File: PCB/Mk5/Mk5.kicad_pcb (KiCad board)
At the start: 2 copper layers, 197 x 253 mm, 40 parts, among them J1 KeyBoard 5,Rd,Ld,D7..0,Gnd, J2 PortB, J3 PortA, J4 COM: Gnd,Rx,Tx,Rts,Dcd,Cts,5v, J5 Conn_01x12, J6 Screw_Terminal_01x02, J7 Conn_01x06_Pin, SW1 SW_Push, U1 74LS92, U10 GAL20V8B-10, U11 GAL20V8B-10, U2 R65C02, U3 CD4059A, U4 EEPROM, U5 62256, U6 MC68B50, U7 R6522, U8 74LS573, U9 DS1813

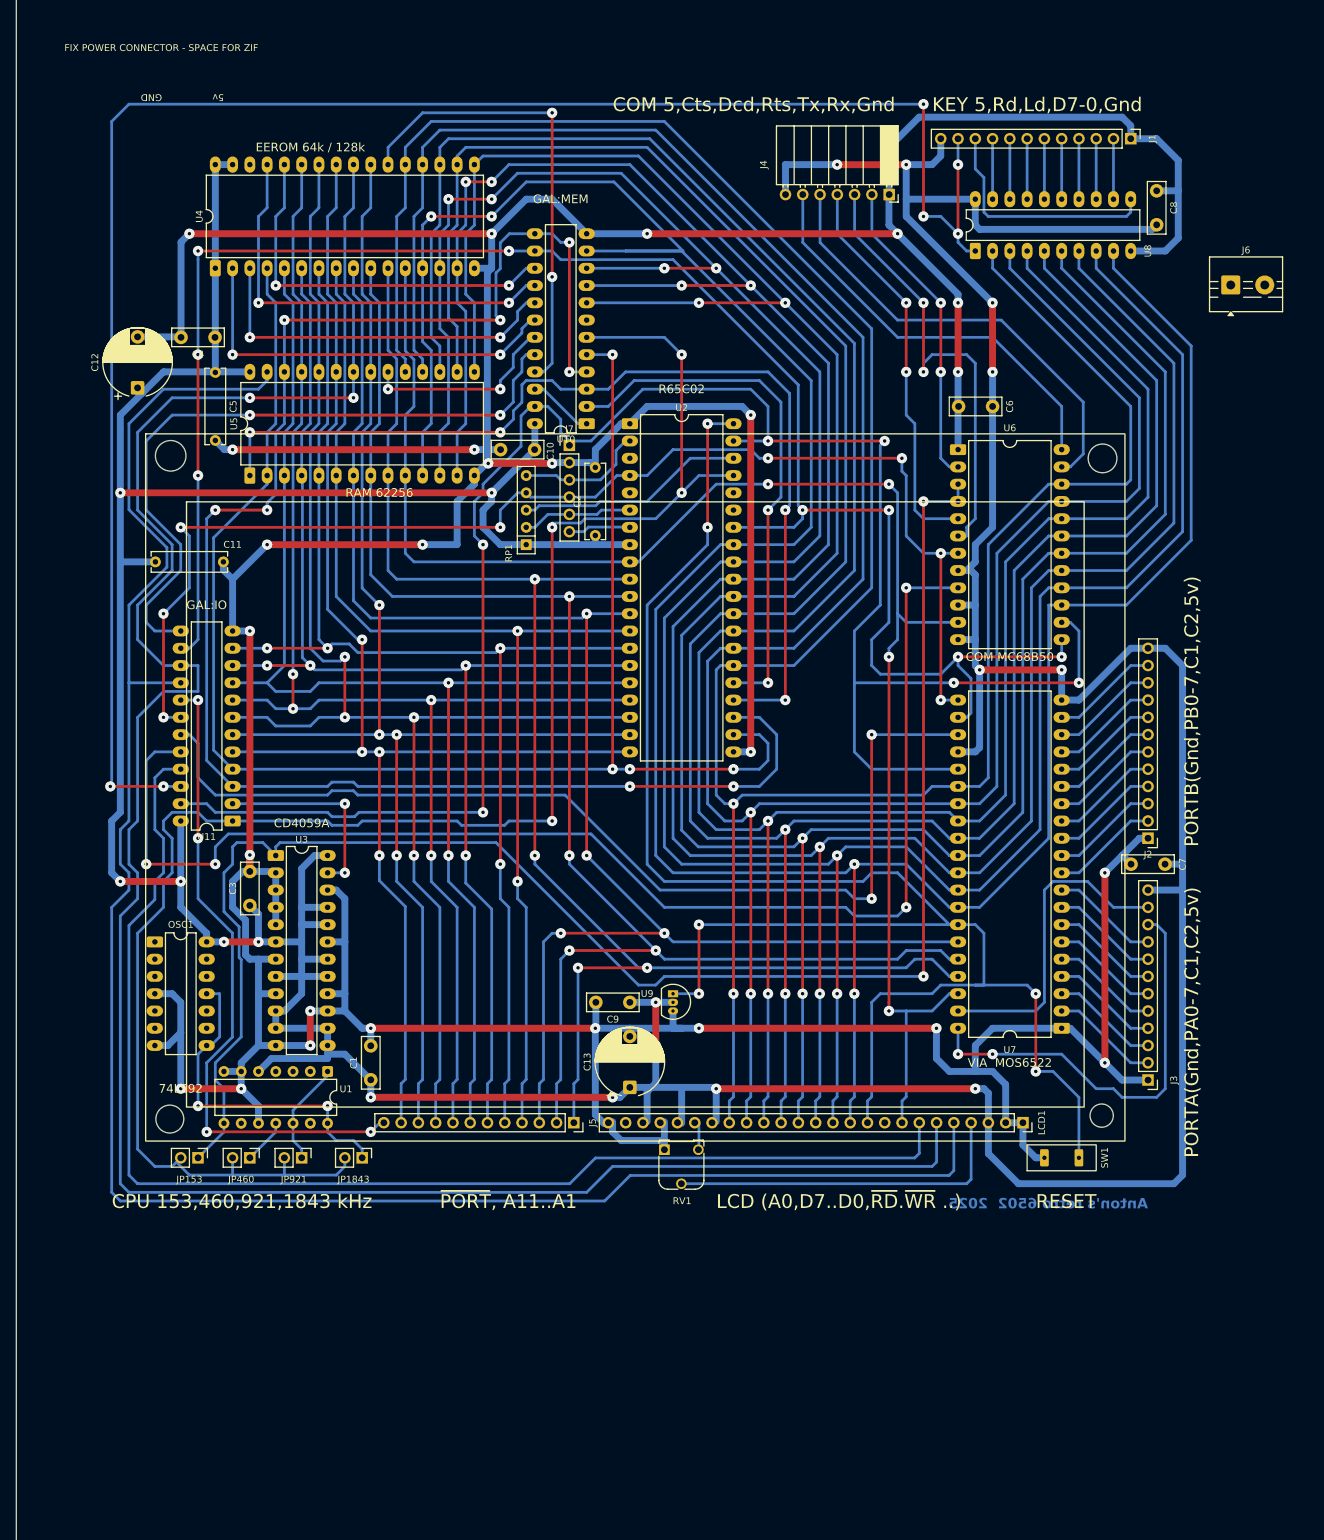
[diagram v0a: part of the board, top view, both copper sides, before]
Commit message: Latest variation
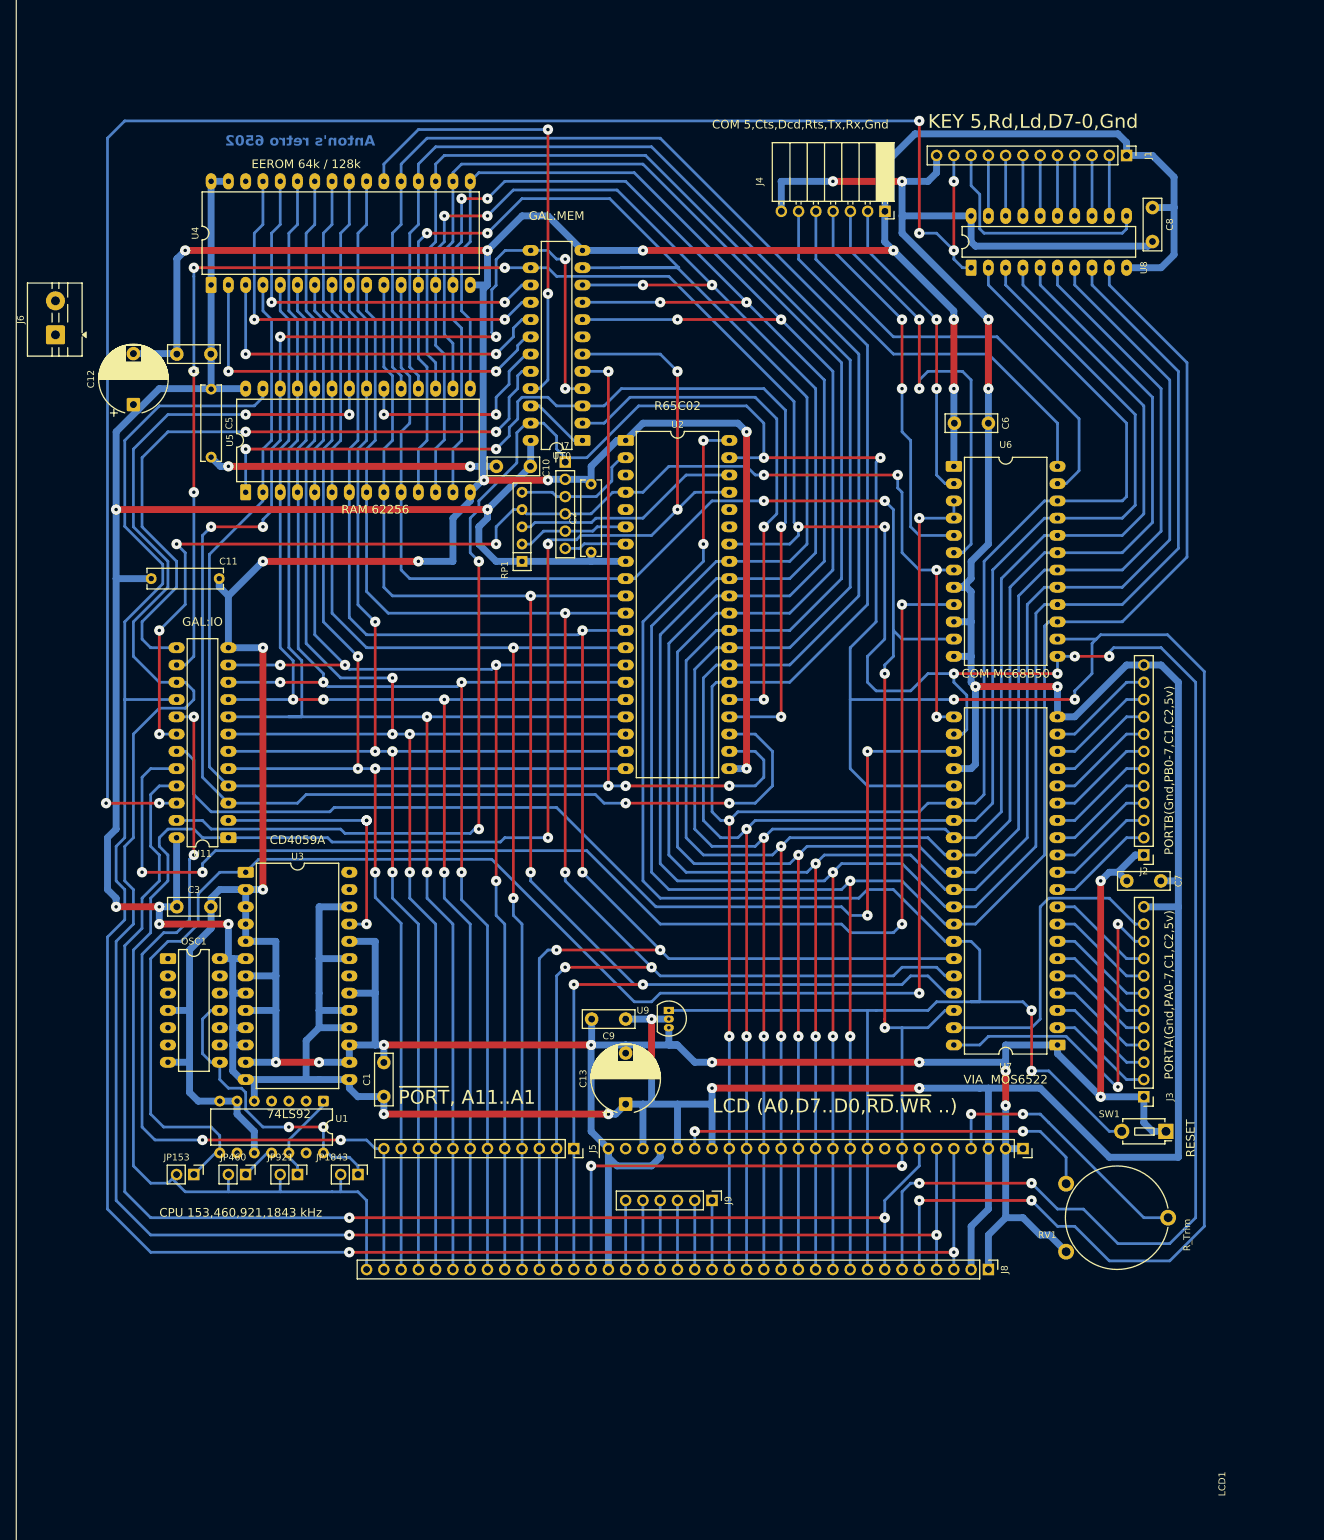
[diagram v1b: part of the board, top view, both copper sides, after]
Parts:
- added J8: Conn_01x37_Pin, Connector_PinHeader_2.54mm:PinHeader_1x37_P2.54mm_Vertical, F.Cu at (152.4, 195.6)
- added J9: Conn_01x06_Pin, Connector_PinHeader_2.54mm:PinHeader_1x06_P2.54mm_Vertical, F.Cu at (111.8, 185.4)
- RV1: footprint Potentiometer_THT:Potentiometer_Runtron_RM-065_Vertical -> Potentiometer_THT:Potentiometer_Piher_PT-15-V15_Vertical
- SW1: value SW_Push -> RST; footprint Library:MiniSwitch -> Button_Switch_THT:SW_PUSH_1P1T_6x3.5mm_H4.3_APEM_MJTP1243
- U3: footprint Package_DIP:DIP-24_W7.62mm_LongPads -> Package_DIP:DIP-26_W15.24mm_LongPads
- moved J6 173.0 mm to (15.2, 58.1), turned to 90 degrees
- moved RV1 60.9 mm to (163.8, 193.0)
- moved LCD1 59.4 mm to (127.0, 177.8)
- moved SW1 15.8 mm to (178.5, 175.3), turned to 180 degrees
- moved C3 10.7 mm to (33.1, 142.2), turned to 0 degrees
- moved U3 5.06 mm to (43.2, 137.2)
- moved U1 4.40 mm to (54.6, 170.8)
- moved J5 3.81 mm to (91.4, 177.8)
- moved OSC1 3.12 mm to (31.8, 149.9)
- moved C1 3.12 mm to (63.5, 170.1)
- moved C7 2.54 mm to (177.8, 138.4)
- moved J2 2.54 mm to (175.3, 134.6)
- moved J3 2.54 mm to (175.3, 170.2)
- moved JP153 2.54 mm to (35.6, 181.6)
- moved JP1843 2.54 mm to (59.7, 181.6)
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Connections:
- net Net-(U10-Clk/In14) renamed /BankWr
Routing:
- net /Clk2: track 287.0 -> 450.0 mm, vias 6 -> 8
- net /R~{W}: track 267.2 -> 429.6 mm, vias 8 -> 12
- net /A0: track 235.3 -> 299.8 mm, vias 4 -> 6
- net Net-(LCD1-VOUT): track 4.20 -> 62.6 mm, vias 0 -> 2
- net GND: track 892.8 -> 941.9 mm
- net +5V: track 822.2 -> 848.1 mm
- net /~{PORT}: track 96.9 -> 121.8 mm
- net /A9: track 209.0 -> 231.3 mm
- net /A6: track 188.3 -> 207.9 mm
- net /A5: track 187.8 -> 207.2 mm
- net /A8: track 205.4 -> 224.3 mm, vias 4 -> 2
- net /D6: track 390.6 -> 409.4 mm
- net /D1: track 424.6 -> 443.3 mm
- net /D7: track 391.9 -> 410.6 mm
- net /D5: track 389.6 -> 408.3 mm
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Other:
- board text added: "Anton's retro 6502"
- board text removed: "5v GND"
- board text removed: "Anton's retro 6502 2025"
- board text removed: "FIX POWER CONNECTOR - SPACE FOR ZIF"
